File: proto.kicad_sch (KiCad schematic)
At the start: 1 part, among them U2 MCP2515_Breakout

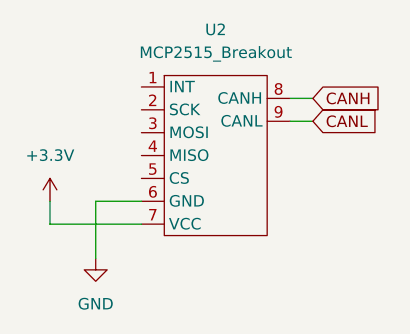
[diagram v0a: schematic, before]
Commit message: More changes
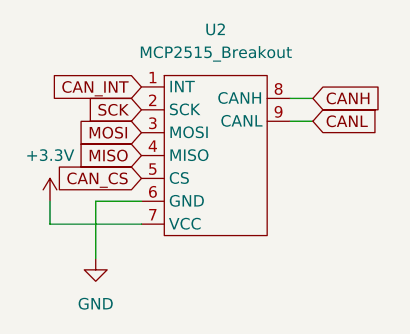
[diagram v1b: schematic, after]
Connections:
- net CAN_INT: now reaches U2.1 (INT)
- net SCK: now reaches U2.2 (SCK)
- net MOSI: now reaches U2.3 (MOSI)
- net MISO: now reaches U2.4 (MISO)
- net CAN_CS: now reaches U2.5 (CS)
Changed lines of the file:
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@@
     (stroke (width 0) (type default) (color 0 0 0 0))
+  )
+  (global_label "CAN_CS" (shape input) (at 33.02 35.56 180) (fields_autoplaced)
+    (effects (font (size 1.27 1.27)) (justify right))
+    (property "Intersheet References" "${INTERSHEET_REFS}" (id 0) (at 23.5596 35.4806 0)
+      (effects (font (size 1.27 1.27)) (justify right) hide)
+    )
   )
   (global_label "CANL" (shape input) (at 52.07 29.21 0) (fields_autoplaced)
@@
     )
   )
+  (global_label "MISO" (shape input) (at 33.02 33.02 180) (fields_autoplaced)
+    (effects (font (size 1.27 1.27)) (justify right))
+    (property "Intersheet References" "${INTERSHEET_REFS}" (id 0) (at 26.0996 32.9406 0)
+      (effects (font (size 1.27 1.27)) (justify right) hide)
+    )
+  )
+  (global_label "SCK" (shape input) (at 33.02 27.94 180) (fields_autoplaced)
+    (effects (font (size 1.27 1.27)) (justify right))
+    (property "Intersheet References" "${INTERSHEET_REFS}" (id 0) (at 26.9463 28.0194 0)
+      (effects (font (size 1.27 1.27)) (justify right) hide)
+    )
+  )
+  (global_label "CAN_INT" (shape input) (at 33.02 25.4 180) (fields_autoplaced)
+    (effects (font (size 1.27 1.27)) (justify right))
+    (property "Intersheet References" "${INTERSHEET_REFS}" (id 0) (at 23.1363 25.3206 0)
+      (effects (font (size 1.27 1.27)) (justify right) hide)
+    )
+  )
+  (global_label "MOSI" (shape input) (at 33.02 30.48 180) (fields_autoplaced)
+    (effects (font (size 1.27 1.27)) (justify right))
+    (property "Intersheet References" "${INTERSHEET_REFS}" (id 0) (at 26.0996 30.4006 0)
+      (effects (font (size 1.27 1.27)) (justify right) hide)
+    )
+  )
